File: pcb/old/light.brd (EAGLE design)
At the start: 15.7 x 15.2 mm, 5 parts, among them J3 FFC3B07-05-T, U1 TEMT6000

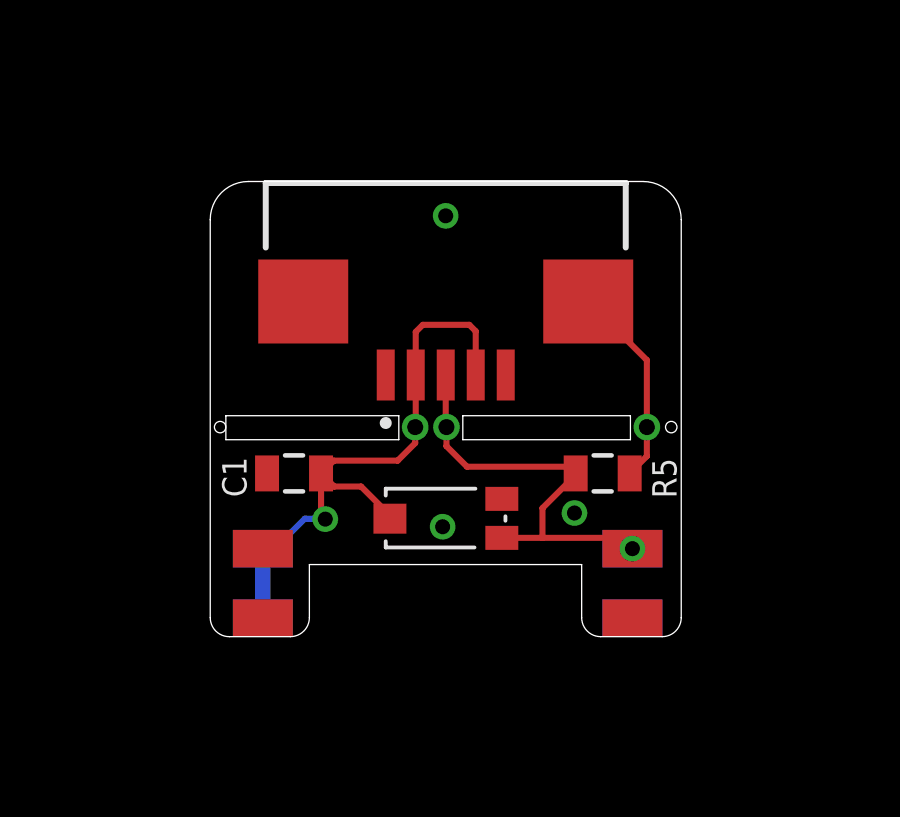
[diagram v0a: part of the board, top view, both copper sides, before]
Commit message: cleanup PCB files
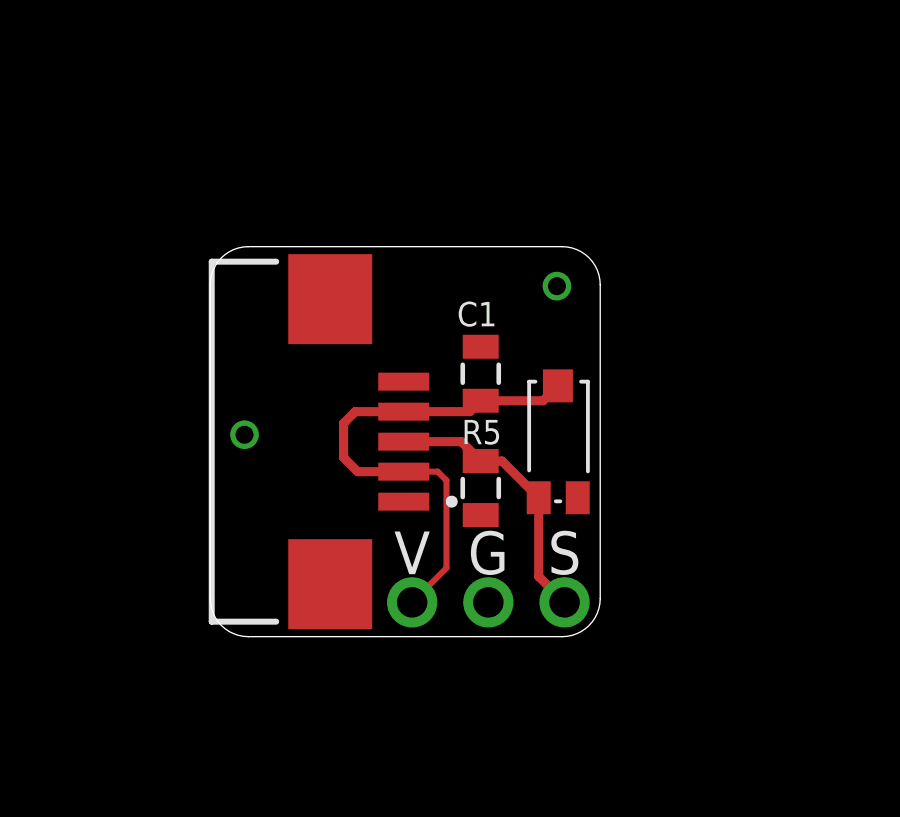
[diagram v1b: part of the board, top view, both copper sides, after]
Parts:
- removed U$1: LS_VERT, apricot:LS_VERT
- added JP1: (no value), adafruit_changed:1X03-CLEANBIG
- moved C1 7.05 mm to (9.02, 8.76), turned to 270 degrees
- moved J3 6.05 mm to (4.00, 6.50), turned to 270 degrees
- moved U1 4.54 mm to (11.6, 6.50), turned to 90 degrees
- moved R5 4.09 mm to (9.02, 4.95), turned to 90 degrees
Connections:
- net +3V3: now also JP1.1; no longer U$1.B1, U$1.B2
- net GND: now also JP1.2; no longer U$1.T1, U$1.T2
- net S: now also JP1.3; no longer U$1.B3, U$1.B4, U$1.T3, U$1.T4
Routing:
- net GND: track 6.78 -> 0.00 mm, vias 4 -> 2
- net S: track 14.4 -> 9.12 mm, vias 2 -> 0
- net +3V3: track 20.3 -> 17.1 mm, vias 2 -> 0
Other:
- board size 15.7 x 15.2 mm -> 13 x 13 mm
- board text added: "G"
- board text added: "PulseHPT.com dekuNukem 2023"
- board text added: "S"
- board text added: "V"
- board text removed: "PulseHPT.com"
